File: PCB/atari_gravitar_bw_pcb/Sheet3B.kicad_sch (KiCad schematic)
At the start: 0 parts

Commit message: Sheet 3B complete
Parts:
- added C1, C10, C109, C11, C12, C126, C13, C14, C15, C18, C19, C2, C20, C21, C22, C25, C26, C3, C37, C4, C40, C41, C42, C43, C45, C46, C47, C48, C49, C5, C50, C51, C52, C53, C54, C55, C56, C57, C58, C59, C6, C60, C61, C62, C63, C7, C8: .1, symbol Device:C
- added C110: 2.2uf 35V, symbol Device:C_Polarized_US
- added C111, C121: 22uf 25V, symbol Device:C_Polarized_US
- added C117, C119, C120: 100uf 35V, symbol Device:C_Polarized_US
- added C23: 100pf, symbol Device:C
- added C24: 39pf, symbol Device:C
- added CR3: 1N914, symbol Device:D
- added CR5, CR7: 1N100, symbol Device:D
- added CR6: BLUE LED, symbol Device:LED
- added CR8: 1N754A, symbol Device:D_Zener
- added E_4: 74LS193, symbol atari:74LS193
- added E_4: 74LS00, symbol atari:74LS00
- added F_3: 74S04, symbol atari:74LS04
- added F_4, H_4: 74LS393, symbol atari:74LS393
- added F_7: 74LS14, symbol atari:74LS14
- added K_3: 74LS74, symbol atari:74LS74
- added L1: 100uh, symbol Device:L
- added L_4: 74LS08, symbol atari:74LS08
- added Q1: 2N3904, Package_TO_SOT_THT:TO-92_Inline, symbol Transistor_BJT:2N3904
- added R107, R23, R55, R71, R82: 1k, symbol Device:R_US
- added R195: 270 1/2W, symbol Device:R_US
- added R22, R40, R41, R72: 10k, symbol Device:R_US
- added R42, R73: 220, symbol Device:R_US
- added R69: 22k, symbol Device:R_US
- added R70: 68k, symbol Device:R_US
- added R_8: TL082, symbol atari:TL082
- added TP-15V1, TP12MHZ1, TP15V1, TP5V1, TP5V2, TP6.8V1, TP6MHZ1, TPGND1, TPGND2, TPGND3, TPGND4, TPGND5, TPGND6, TPPHI01, TPRESET1, TP~{RESET}1: tp_2_pin, symbol atari:tp_2_pin
- added VR1: L7915, symbol atari:L7915
- added VR2: L7815, symbol atari:L7815
- added Y1: 12.096MHz, symbol Device:Crystal
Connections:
- new net: C23.1, Q1.2 (B), R40.1, R41.2, Y1.2
- new net: R70.2, R71.1, R73.1, R_8.1
- new net: R69.2, R70.1, R72.2, R_8.3 (+)
- new net: CR6.2 (A), R107.2
- new net: C23.2, C24.1, F_3.11, L1.1, Q1.1 (E)
- new net: L1.2, R42.1
- new net: K_3.2 (D), L_4.8
- new net: CR3.2 (A), F_7.3, R71.2, TPRESET1.1, TPRESET1.2
- new net: H_4.6 (1QD), K_3.3 (C)
- new net: E_4.7 (QD), F_4.13 (2CK)
- new net: E_4.3, H_4.12 (2CLR), H_4.2 (1CLR)
- new net: H_4.1 (1CK), H_4.8 (2QD)
- new net: F_4.1 (1CK), F_4.8 (2QD)
- new net +10V: C55.1, R72.1, R_8.8 (V+)
- new net +15V: C121.1, CR7.1 (K), R195.1, TP15V1.1, TP15V1.2, VR2.3 (OUT)
- new net +24V: C120.1, VR2.1 (IN)
- new net +5V: C1.1, C10.1, C109.1, C11.1, C117.1, C12.1, C13.1, C14.1, C15.1, C18.1, C19.1, C2.1, C20.1, C21.1, C22.2, C25.1, C26.1, C3.1, C37.1, C4.1, C40.1, C41.1, C42.1, C43.1, C45.1, C46.1, C47.1, C48.1, C49.1, C5.1, C50.1, C51.1, C52.1, C53.1, C54.1, C56.1, C57.1, C58.1, C59.1, C6.1, C60.1, C61.1, C62.1, C63.1, C7.1, C8.1, CR3.1 (K), E_4.16 (VCC), F_4.14 (VCC), H_4.14 (VCC), K_3.14 (VCC), Q1.3 (C), R107.1, R22.1, R23.2, R41.1, R55.2, R82.2, R_8.2 (-), TP5V1.1, TP5V1.2, TP5V2.1, TP5V2.2
- new net +6V: C126.1, CR8.1 (K), R195.2, TP6.8V1.1, TP6.8V1.2
- new net -15V: C111.2, CR5.2 (A), TP-15V1.1, TP-15V1.2, VR1.3 (VO)
- new net -24V: C110.2, C119.2, VR1.2 (VI)
- new net 1.5MHZ: E_4.6 (QC), TPPHI01.1, TPPHI01.2
- new net 12KHZ: F_4.4 (1QB)
- new net 12MHZ: E_4.5 (D2), F_3.10, TP12MHZ1.1, TP12MHZ1.2
- new net 3KHZ: F_4.6 (1QD), H_4.13 (2CK)
- new net 3MHZ: E_4.2 (QB)
- new net 6MHZ: E_4.3 (QA), TP6MHZ1.1, TP6MHZ1.2
- new net GND: C1.2, C10.2, C109.2, C11.2, C110.1, C111.1, C117.2, C119.1, C12.2, C120.2, C121.2, C126.2, C13.2, C14.2, C15.2, C18.2, C19.2, C2.2, C20.2, C21.2, C22.1, C24.2, C25.2, C26.2, C3.2, C37.2, C4.2, C40.2, C41.2, C42.2, C43.2, C45.2, C46.2, C47.2, C48.2, C49.2, C5.2, C50.2, C51.2, C52.2, C53.2, C54.2, C55.2, C56.2, C57.2, C58.2, C59.2, C6.2, C60.2, C61.2, C62.2, C63.2, C7.2, C8.2, CR5.1 (K), CR6.1 (K), CR7.2 (A), CR8.2 (A), E_4.8 (GND), F_4.7 (GND), H_4.7 (GND), K_3.7 (GND), L_4.10, R40.2, R42.2, R69.1, R73.2, R_8.4 (V-), TPGND1.1, TPGND1.2, TPGND2.1, TPGND2.2, TPGND3.1, TPGND3.2, TPGND4.1, TPGND4.2, TPGND5.1, TPGND5.2, TPGND6.1, TPGND6.2, TP~{RESET}1.1, TP~{RESET}1.2, VR1.1 (GND), VR2.2 (GND), Y1.1
- new net POR: E_4.14 (C), F_4.12 (2CLR), F_4.2 (1CLR), F_7.4, F_7.5
- new net PR23: E_4.1 (B), E_4.10 (C), E_4.11 (LD), E_4.15 (A), E_4.4 (D1), E_4.9 (D), K_3.1 (~{R}), R23.1
- new net PR55: R55.1
- new net PR82: R82.1
- new net ~{POR}: E_4.2, F_7.6, K_3.4 (~{S})
- new net ~{RESET}: K_3.6 (~{Q})
- new net ~{WDCLR}: E_4.1
- new net ~{WDDIS}: L_4.9, R22.2
- no-connect marks 0 -> 8
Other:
- note added: "CLOCK"
- note added: "POWER INPUT"
- note added: "POWER-ON RESET"
- note added: "WATCHDOG"

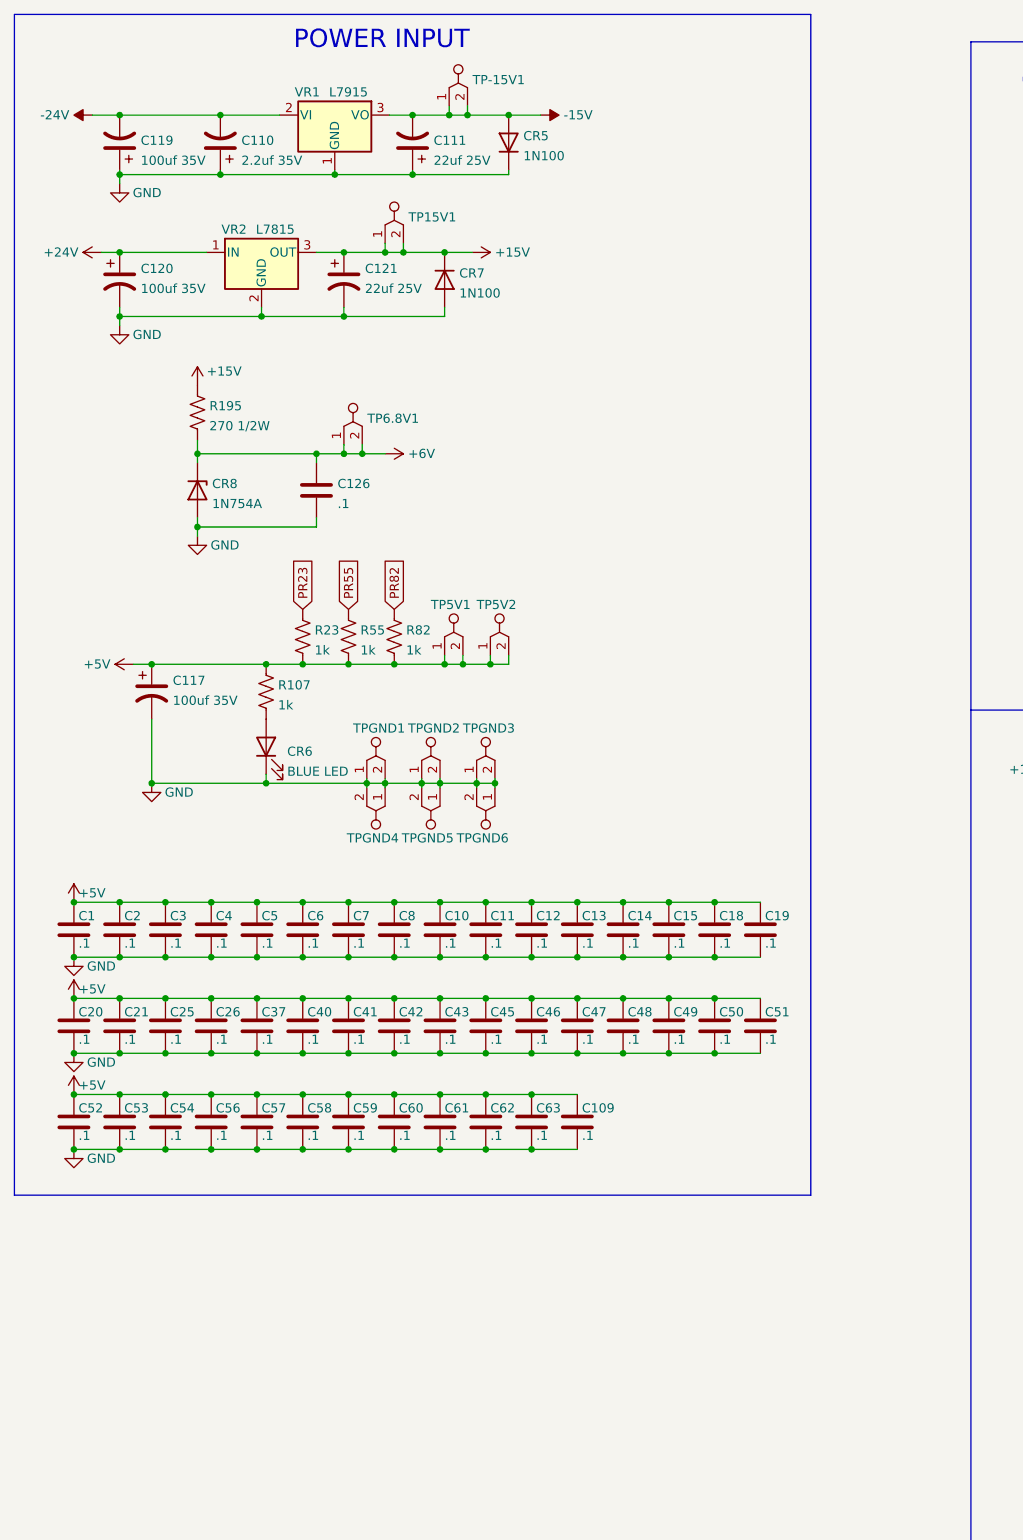
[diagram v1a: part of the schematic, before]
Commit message: Worked on the schematic library
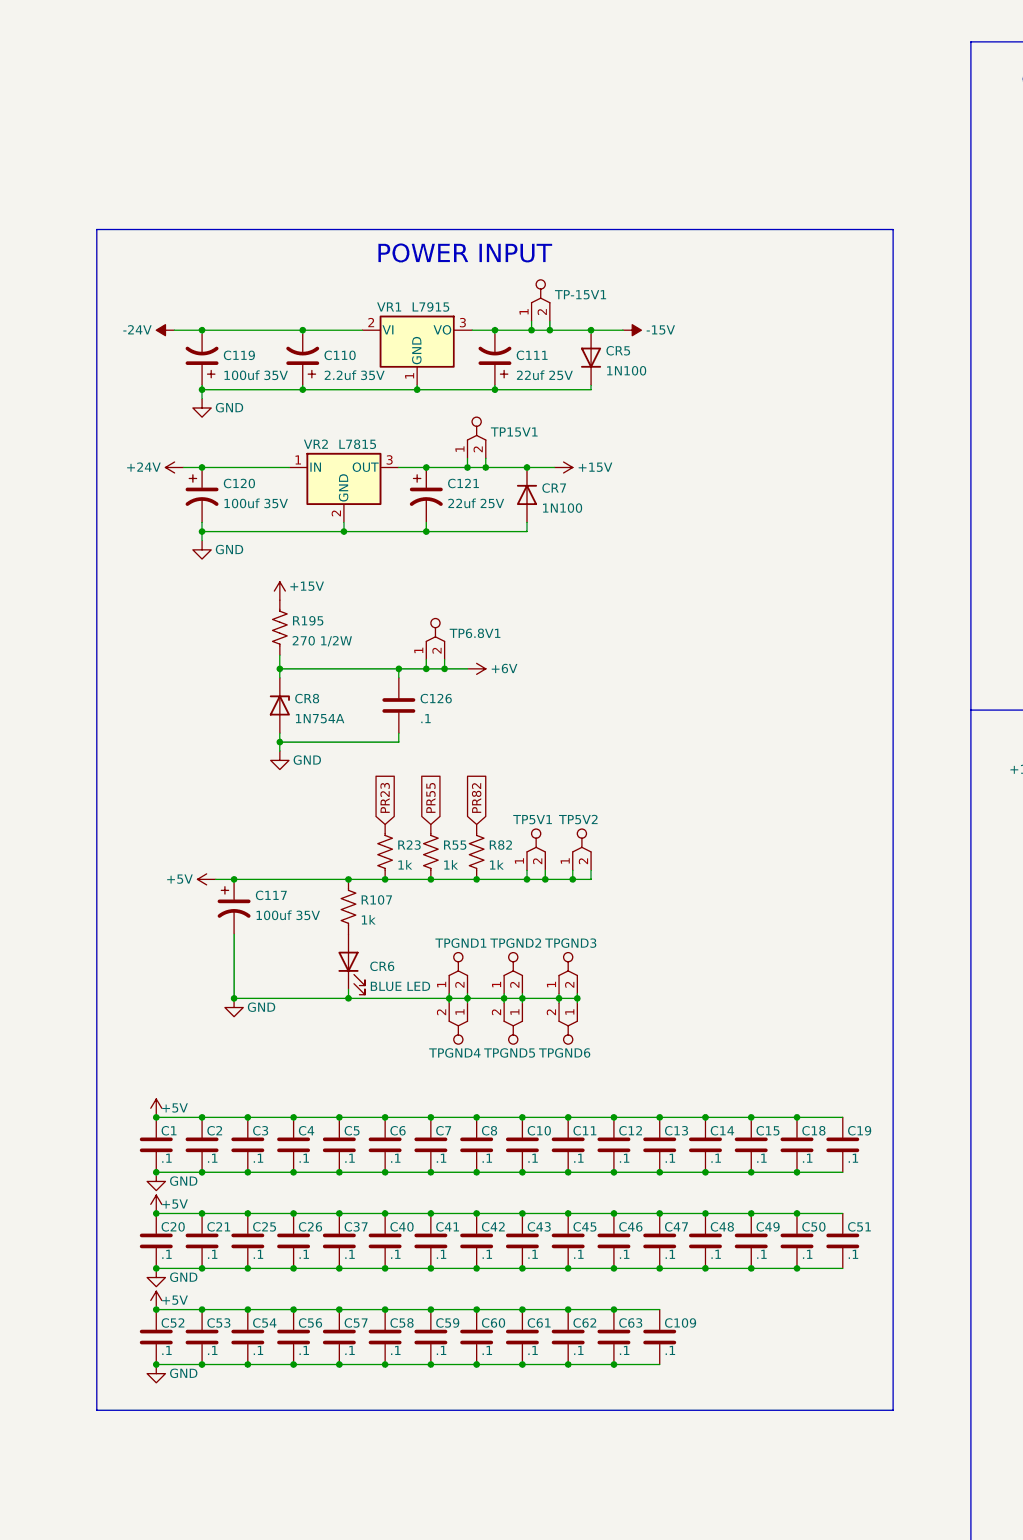
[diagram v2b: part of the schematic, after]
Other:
- moved on the sheet: C1, C10, C109, C11, C110, C111, C117, C119, C12, C120, C121, C126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
